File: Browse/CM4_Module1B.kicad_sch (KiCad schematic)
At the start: 10 parts, among them J3 179-UJ20CHC4SMTTR

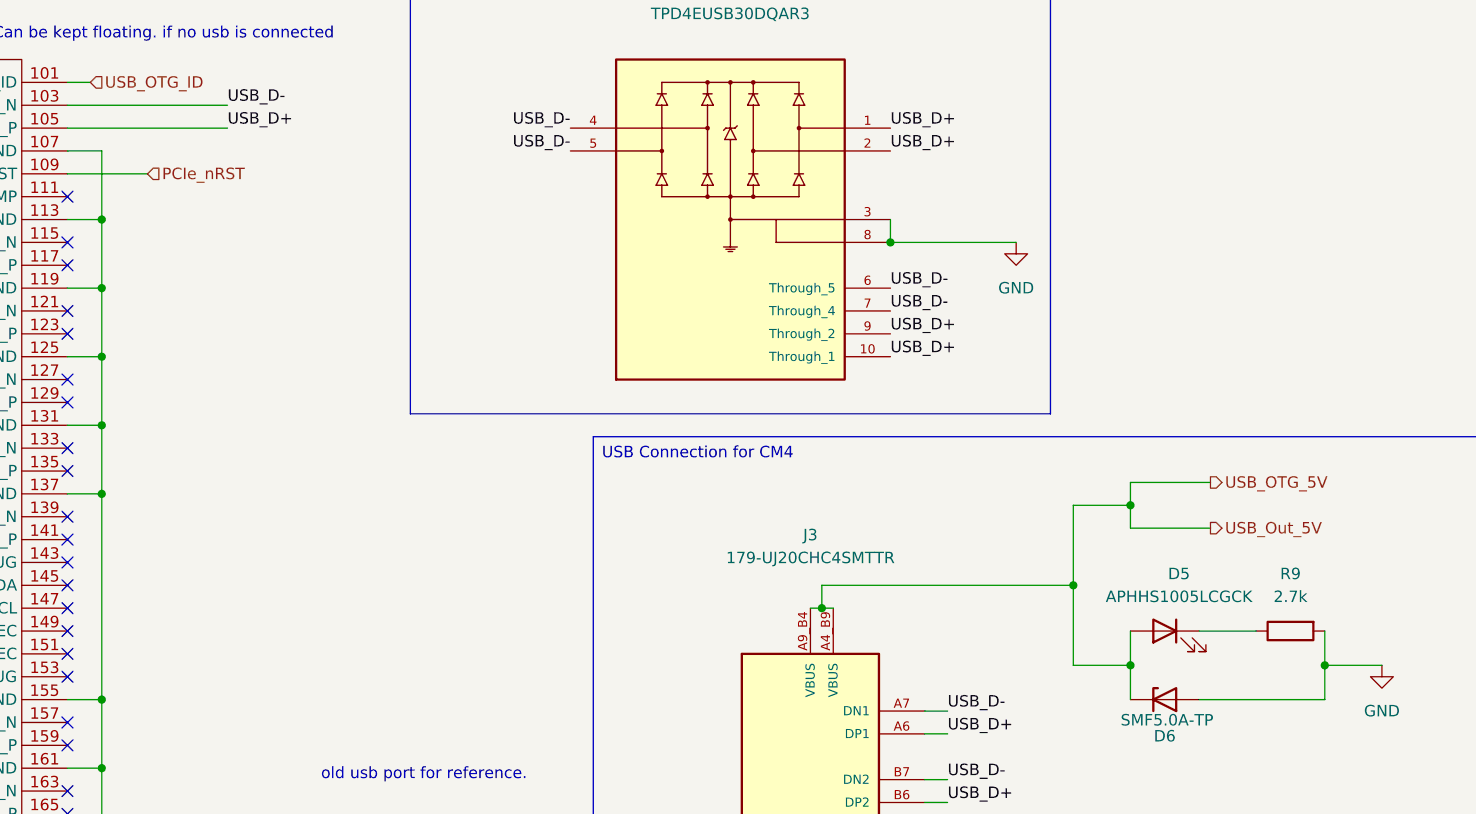
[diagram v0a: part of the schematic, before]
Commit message: Deploying to gh-pages from @ Nautilus-UUV/nautilus-mainboard-PCB@8b02e89ade7c168188296ba6f0516f3abec9166b 🚀
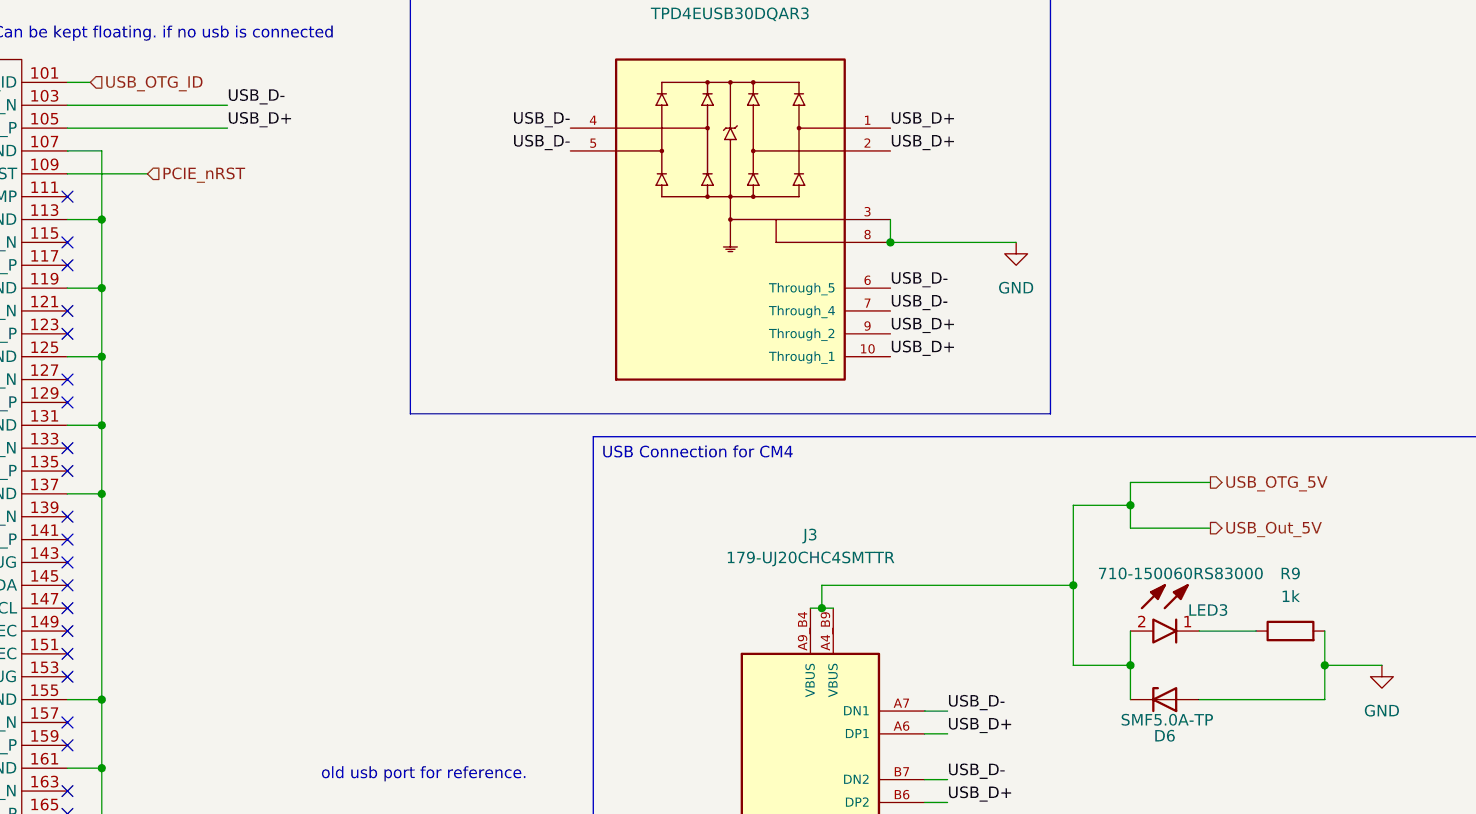
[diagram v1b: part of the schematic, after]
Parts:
- removed D5: APHHS1005LCGCK, LED_SMD:LED_0402_1005Metric, symbol #dzdb:s_dio/D-KIN-APHHS1005LCGCK
- removed R9: 2.7k, Resistor_SMD:R_0603_1608Metric, symbol #dzdb:g_res/R-2.7k-0603
- added LED3: 710-150060RS83000, dz_dio:Wuerth_LED_150060RS83000, symbol #dzdb:s_dio/D-WURT-710-150060RS83000
- added R9: 1k, Resistor_SMD:R_0603_1608Metric, symbol #dzdb:g_res/R-1k-0603
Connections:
- net GND: now also R9.2
- net USB_OTG_5V: now also LED3.2 (A)
- net PCIe_nRST renamed PCIE_nRST
- new net: LED3.1 (K), R9.1
